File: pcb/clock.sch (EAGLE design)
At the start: 27 parts, among them IC1 STM32F072C8T6, IC3 24C64ST

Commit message: USBC, GPS etc
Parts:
- added CONN1: USB-C_WURTH_632723X00011USB-C, breakouts:USB-C_WURTH_632723X00011USB-C
- added SD1: TF-HOLDER, basicBoard:TF-HOLDER
- added U$7: MAX-M8, ubloxLib:MAX-M8
- added U$8: TEMT6000, ProtoSnap-v14a:TEMT6000
- added U$9: DS18B20, DS18B20U:DS18B20
- added X1: (no value), clock:SMACONNECTOR
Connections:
- new net N$4: U$7.11_RF_IN, X1.ANT
- net GND: now also CONN1.GND0, CONN1.GND1, CONN1.GND3, CONN1.GND4, CONN1.SHIELD1, CONN1.SHIELD2, CONN1.SHIELD3, CONN1.SHIELD4, CONN1.SHIELD5, CONN1.SHIELD6, U$7.10_GND, U$7.12_GND, X1.GND1, X1.GND2, X1.GND3, X1.GND4

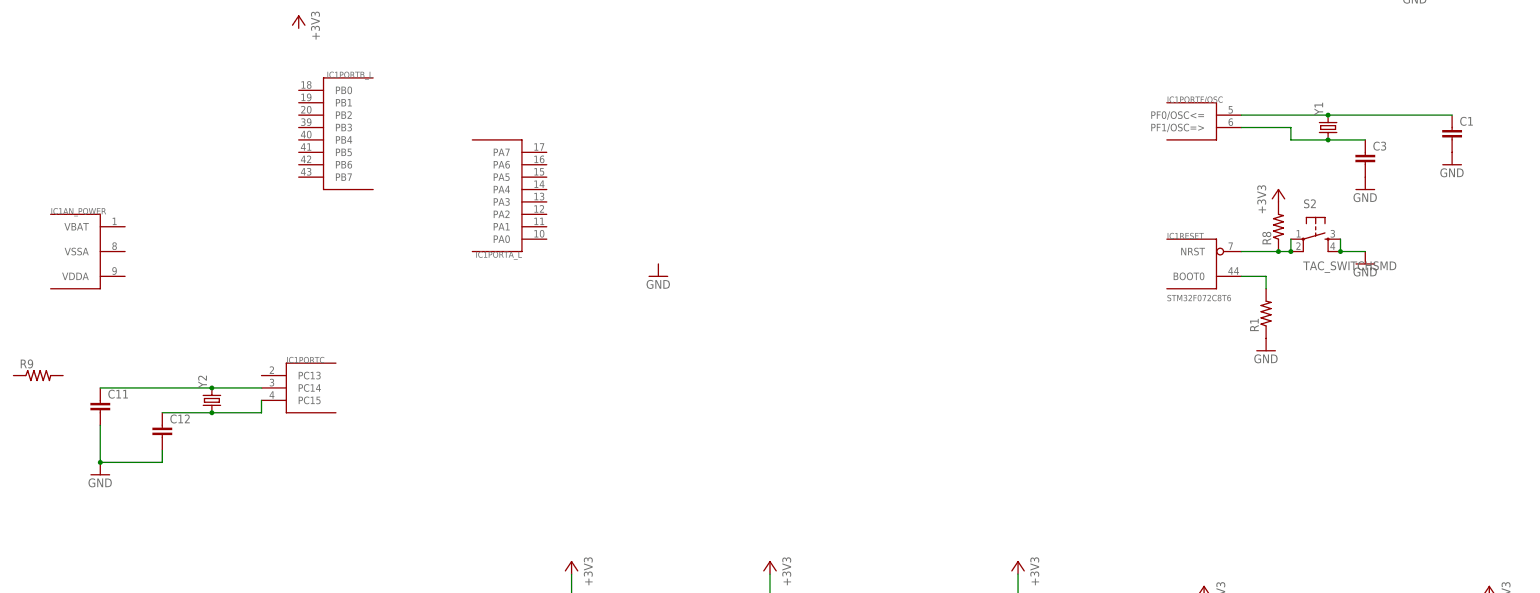
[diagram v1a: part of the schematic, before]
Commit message: added bake control
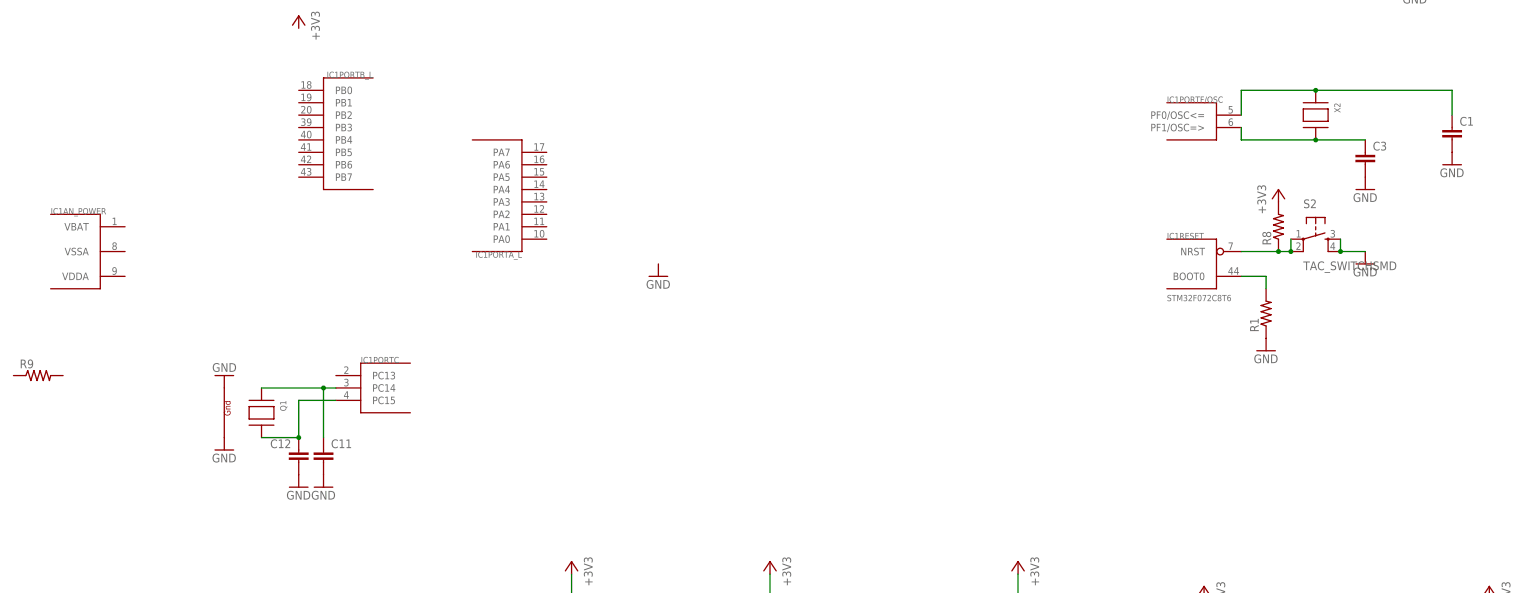
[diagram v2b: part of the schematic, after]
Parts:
- removed Y1: (no value), backplane:CRYSTALHC49US
- removed Y2: (no value), backplane:CRYSTALTC26H_EZ
- added Q1: (no value), adafruit:XTAL-4-3225
- added X2: (no value), adafruit:XTAL-3.2X1.5
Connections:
- net GND: now also Q1.G1, Q1.G2
- net N$1: now also Q1.X1; no longer Y2.2
- net N$2: now also Q1.X2; no longer Y2.1
- net N$6: now also C3.1, IC1PORTF/OSC.PF1/OSC=>, X2.P$2; no longer C1.1, IC1PORTF/OSC.PF0/OSC<=, Y1.2
- net N$7: now also C1.1, IC1PORTF/OSC.PF0/OSC<=, X2.P$1; no longer C3.1, IC1PORTF/OSC.PF1/OSC=>, Y1.1
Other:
- moved on the sheet: C11, C12, IC1PORTC
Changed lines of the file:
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@@
 <part name="C1" library="backplane" deviceset="CAP" device="0805"/>
 <part name="C2" library="backplane" deviceset="C-US" device="C1210"/>
-<part name="Y1" library="backplane" deviceset="CRYSTAL" device="HC49US"/>
 <part name="GND2" library="backplane" deviceset="GND" device=""/>
 <part name="GND3" library="backplane" deviceset="GND" device=""/>
@@
 <part name="+3V14" library="backplane" deviceset="+3V3" device=""/>
 <part name="GND18" library="backplane" deviceset="GND" device=""/>
-<part name="Y2" library="backplane" deviceset="CRYSTAL" device="TC26H_EZ"/>
 <part name="C11" library="backplane" deviceset="CAP" device="0805"/>
 <part name="C12" library="backplane" deviceset="CAP" device="0805"/>
@@
 <part name="GND25" library="backplane" deviceset="GND" device=""/>
 <part name="SD1" library="basicBoard" deviceset="TF-HOLDER" device=""/>
+<part name="Q1" library="adafruit" deviceset="XTAL-4" device="-3225"/>
+<part name="X2" library="adafruit" deviceset="XTAL" device="-3.2X1.5"/>
+<part name="GND26" library="backplane" deviceset="GND" device=""/>
+<part name="GND27" library="backplane" deviceset="GND" device=""/>
+<part name="GND28" library="backplane" deviceset="GND" device=""/>
 </parts>
 <sheets>
@@
 <instance part="C1" gate="G$1" x="190.5" y="-83.82"/>
 <instance part="C2" gate="G$1" x="182.88" y="-43.18"/>
-<instance part="Y1" gate="G$1" x="165.1" y="-81.28" rot="R90"/>
 <instance part="GND2" gate="1" x="172.72" y="-109.22"/>
 <instance part="GND3" gate="1" x="-93.98" y="111.76"/>
@@
 <instance part="+3V14" gate="G$1" x="-223.52" y="58.42"/>
 <instance part="GND18" gate="1" x="-223.52" y="35.56"/>
-<instance part="Y2" gate="G$1" x="-63.5" y="-137.16" rot="R90"/>
-<instance part="C11" gate="G$1" x="-86.36" y="-139.7"/>
-<instance part="C12" gate="G$1" x="-73.66" y="-144.78"/>
-<instance part="GND19" gate="1" x="-86.36" y="-152.4"/>
+<instance part="C11" gate="G$1" x="-40.64" y="-149.86"/>
+<instance part="C12" gate="G$1" x="-45.72" y="-149.86" rot="MR0"/>
+<instance part="GND19" gate="1" x="-60.96" y="-147.32"/>
 <instance part="R8" gate="G$1" x="154.94" y="-101.6" rot="R90"/>
 <instance part="+3V15" gate="G$1" x="154.94" y="-93.98"/>
@@
 <instance part="IC1" gate="PORTB_H" x="-76.2" y="-43.18" rot="R270"/>
 <instance part="IC1" gate="POWER" x="-76.2" y="137.16"/>
-<instance part="IC1" gate="PORTC" x="-45.72" y="-134.62"/>
+<instance part="IC1" gate="PORTC" x="-30.48" y="-134.62"/>
 <instance part="IC1" gate="PORTF/OSC" x="139.7" y="-78.74"/>
 <instance part="IC1" gate="AN_POWER" x="-91.44" y="-106.68"/>
@@
 <instance part="GND25" gate="1" x="426.72" y="-170.18"/>
 <instance part="SD1" gate="G$1" x="391.16" y="-205.74"/>
+<instance part="Q1" gate="G$1" x="-53.34" y="-139.7" rot="R270"/>
+<instance part="X2" gate="G$1" x="162.56" y="-78.74" rot="R270"/>
+<instance part="GND26" gate="1" x="-45.72" y="-154.94"/>
+<instance part="GND27" gate="1" x="-40.64" y="-154.94"/>
+<instance part="GND28" gate="1" x="-60.96" y="-132.08" rot="R180"/>
 </instances>
 <busses>
@@
 <pinref part="U$6" gate="G$1" pin="GND"/>
 <pinref part="GND16" gate="1" pin="GND"/>
-</segment>
-<segment>
-<pinref part="C11" gate="G$1" pin="2"/>
-<pinref part="GND19" gate="1" pin="GND"/>
-<wire x1="-86.36" y1="-142.24" x2="-86.36" y2="-149.86" width="0.1524" layer="91"/>
-<pinref part="C12" gate="G$1" pin="2"/>
-<wire x1="-86.36" y1="-149.86" x2="-73.66" y2="-149.86" width="0.1524" layer="91"/>
-<wire x1="-73.66" y1="-149.86" x2="-73.66" y2="-147.32" width="0.1524" layer="91"/>
-<junction x="-86.36" y="-149.86"/>
 </segment>
 <segment>
@@
 <junction x="426.72" y="-167.64"/>
 </segment>
+<segment>
+<pinref part="C12" gate="G$1" pin="2"/>
+<pinref part="GND26" gate="1" pin="GND"/>
+</segment>
+<segment>
+<pinref part="C11" gate="G$1" pin="2"/>
+<pinref part="GND27" gate="1" pin="GND"/>
+</segment>
+<segment>
+<pinref part="Q1" gate="G$1" pin="G2"/>
+<pinref part="GND19" gate="1" pin="GND"/>
+</segment>
+<segment>
+<pinref part="Q1" gate="G$1" pin="G1"/>
+<pinref part="GND28" gate="1" pin="GND"/>
+</segment>
 </net>
 <net name="+3V3" class="0">
@@
 </segment>
 </net>
-<net name="N$1" class="0">
-<segment>
-<pinref part="Y2" gate="G$1" pin="2"/>
-<pinref part="IC1" gate="PORTC" pin="PC14"/>
-<wire x1="-63.5" y1="-134.62" x2="-53.34" y2="-134.62" width="0.1524" layer="91"/>
-<pinref part="C11" gate="G$1" pin="1"/>
-<wire x1="-86.36" y1="-134.62" x2="-63.5" y2="-134.62" width="0.1524" layer="91"/>
-<junction x="-63.5" y="-134.62"/>
-</segment>
-</net>
-<net name="N$2" class="0">
-<segment>
-<pinref part="IC1" gate="PORTC" pin="PC15"/>
-<wire x1="-53.34" y1="-137.16" x2="-53.34" y2="-139.7" width="0.1524" layer="91"/>
-<pinref part="Y2" gate="G$1" pin="1"/>
-<wire x1="-53.34" y1="-139.7" x2="-63.5" y2="-139.7" width="0.1524" layer="91"/>
-<pinref part="C12" gate="G$1" pin="1"/>
-<wire x1="-63.5" y1="-139.7" x2="-73.66" y2="-139.7" width="0.1524" layer="91"/>
-<junction x="-63.5" y="-139.7"/>
-</segment>
-</net>
 <net name="N$3" class="0">
 <segment>
@@
 </segment>
 </net>
-<net name="N$6" class="0">
-<segment>
-<pinref part="IC1" gate="PORTF/OSC" pin="PF0/OSC&lt;="/>
-<pinref part="Y1" gate="G$1" pin="2"/>
-<wire x1="147.32" y1="-78.74" x2="165.1" y2="-78.74" width="0.1524" layer="91"/>
-<pinref part="C1" gate="G$1" pin="1"/>
-<wire x1="165.1" y1="-78.74" x2="190.5" y2="-78.74" width="0.1524" layer="91"/>
-<junction x="165.1" y="-78.74"/>
-</segment>
-</net>
-<net name="N$7" class="0">
-<segment>
-<pinref part="IC1" gate="PORTF/OSC" pin="PF1/OSC=&gt;"/>
-<wire x1="147.32" y1="-81.28" x2="157.48" y2="-81.28" width="0.1524" layer="91"/>
-<wire x1="157.48" y1="-81.28" x2="157.48" y2="-83.82" width="0.1524" layer="91"/>
-<pinref part="Y1" gate="G$1" pin="1"/>
-<wire x1="157.48" y1="-83.82" x2="165.1" y2="-83.82" width="0.1524" layer="91"/>
-<pinref part="C3" gate="G$1" pin="1"/>
-<wire x1="165.1" y1="-83.82" x2="172.72" y2="-83.82" width="0.1524" layer="91"/>
-<junction x="165.1" y="-83.82"/>
-</segment>
-</net>
 <net name="N$4" class="0">
 <segment>
@@
 </segment>
 </net>
+<net name="N$6" class="0">
+<segment>
+<pinref part="IC1" gate="PORTF/OSC" pin="PF1/OSC=&gt;"/>
+<pinref part="X2" gate="G$1" pin="P$2"/>
+<wire x1="147.32" y1="-81.28" x2="147.32" y2="-83.82" width="0.1524" layer="91"/>
+<wire x1="147.32" y1="-83.82" x2="162.56" y2="-83.82" width="0.1524" layer="91"/>
+<pinref part="C3" gate="G$1" pin="1"/>
+<wire x1="162.56" y1="-83.82" x2="172.72" y2="-83.82" width="0.1524" layer="91"/>
+<junction x="162.56" y="-83.82"/>
+</segment>
+</net>
+<net name="N$7" class="0">
+<segment>
+<pinref part="IC1" gate="PORTF/OSC" pin="PF0/OSC&lt;="/>
+<pinref part="X2" gate="G$1" pin="P$1"/>
+<wire x1="147.32" y1="-78.74" x2="147.32" y2="-73.66" width="0.1524" layer="91"/>
+<wire x1="147.32" y1="-73.66" x2="162.56" y2="-73.66" width="0.1524" layer="91"/>
+<pinref part="C1" gate="G$1" pin="1"/>
+<wire x1="162.56" y1="-73.66" x2="190.5" y2="-73.66" width="0.1524" layer="91"/>
+<wire x1="190.5" y1="-73.66" x2="190.5" y2="-78.74" width="0.1524" layer="91"/>
+<junction x="162.56" y="-73.66"/>
+</segment>
+</net>
+<net name="N$1" class="0">
+<segment>
+<pinref part="IC1" gate="PORTC" pin="PC14"/>
+<pinref part="Q1" gate="G$1" pin="X1"/>
+<wire x1="-38.1" y1="-134.62" x2="-40.64" y2="-134.62" width="0.1524" layer="91"/>
+<pinref part="C11" gate="G$1" pin="1"/>
+<wire x1="-40.64" y1="-134.62" x2="-53.34" y2="-134.62" width="0.1524" layer="91"/>
+<wire x1="-40.64" y1="-144.78" x2="-40.64" y2="-134.62" width="0.1524" layer="91"/>
+<junction x="-40.64" y="-134.62"/>
+</segment>
+</net>
+<net name="N$2" class="0">
+<segment>
+<pinref part="IC1" gate="PORTC" pin="PC15"/>
+<wire x1="-38.1" y1="-137.16" x2="-45.72" y2="-137.16" width="0.1524" layer="91"/>
+<wire x1="-45.72" y1="-137.16" x2="-45.72" y2="-144.78" width="0.1524" layer="91"/>
+<pinref part="Q1" gate="G$1" pin="X2"/>
+<wire x1="-45.72" y1="-144.78" x2="-53.34" y2="-144.78" width="0.1524" layer="91"/>
+<pinref part="C12" gate="G$1" pin="1"/>
+<junction x="-45.72" y="-144.78"/>
+</segment>
+</net>
